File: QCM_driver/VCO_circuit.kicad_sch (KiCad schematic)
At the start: 31 parts, among them Q1 BC817-25

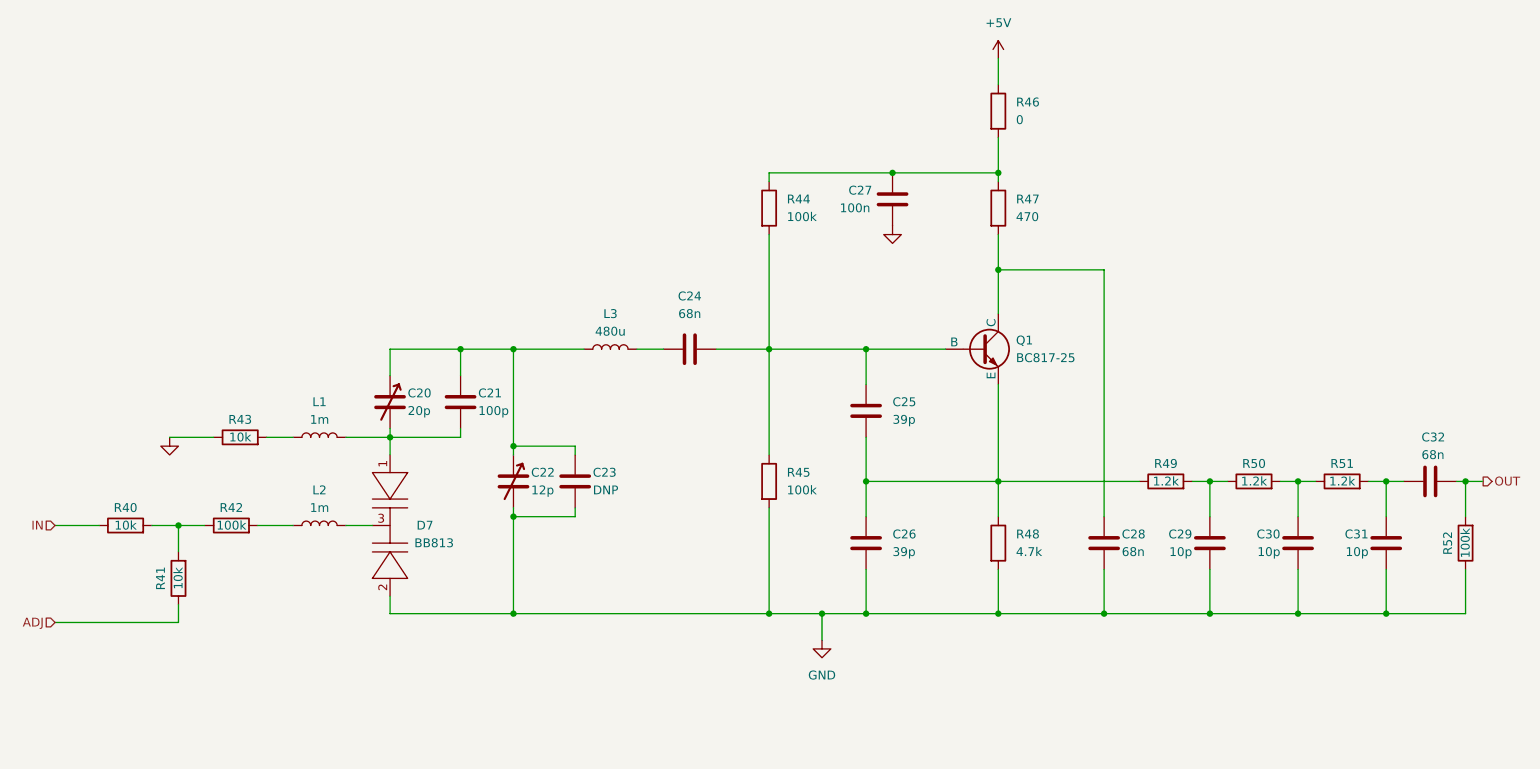
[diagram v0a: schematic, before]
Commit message: PCB and schematic V1.0
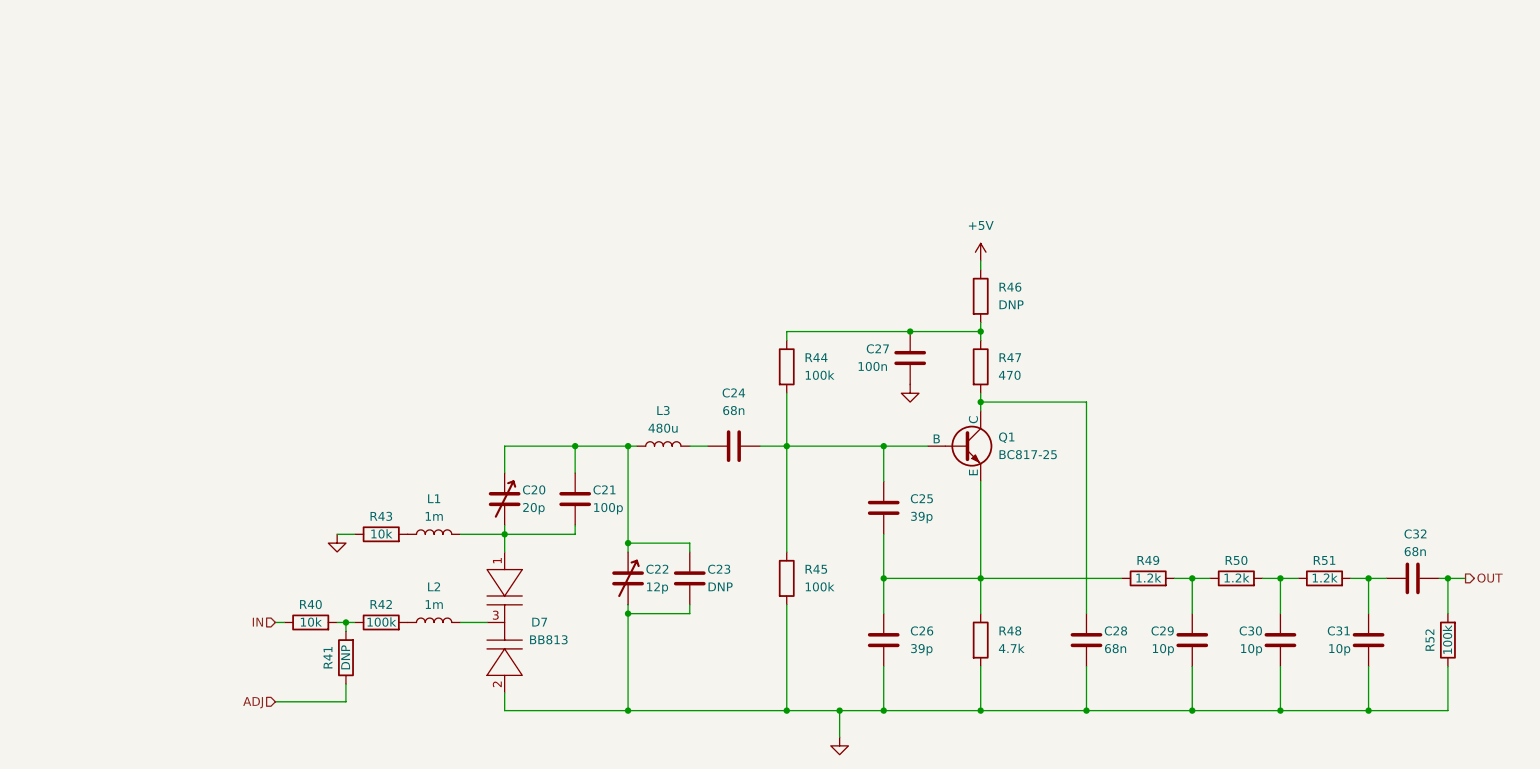
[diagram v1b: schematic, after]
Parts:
- R41: value 10k -> DNP
- R46: value 0 -> DNP
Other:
- moved on the sheet: C20, C21, C22, C23, C24, C25, C26, C27, C28, C29, C30, C31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
